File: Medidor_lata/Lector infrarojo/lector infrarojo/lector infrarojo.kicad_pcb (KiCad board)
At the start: 2 copper layers, 70 x 23 mm, 22 parts, among them J1 Conn_01x02_Female, J2 Conn_01x02_Female

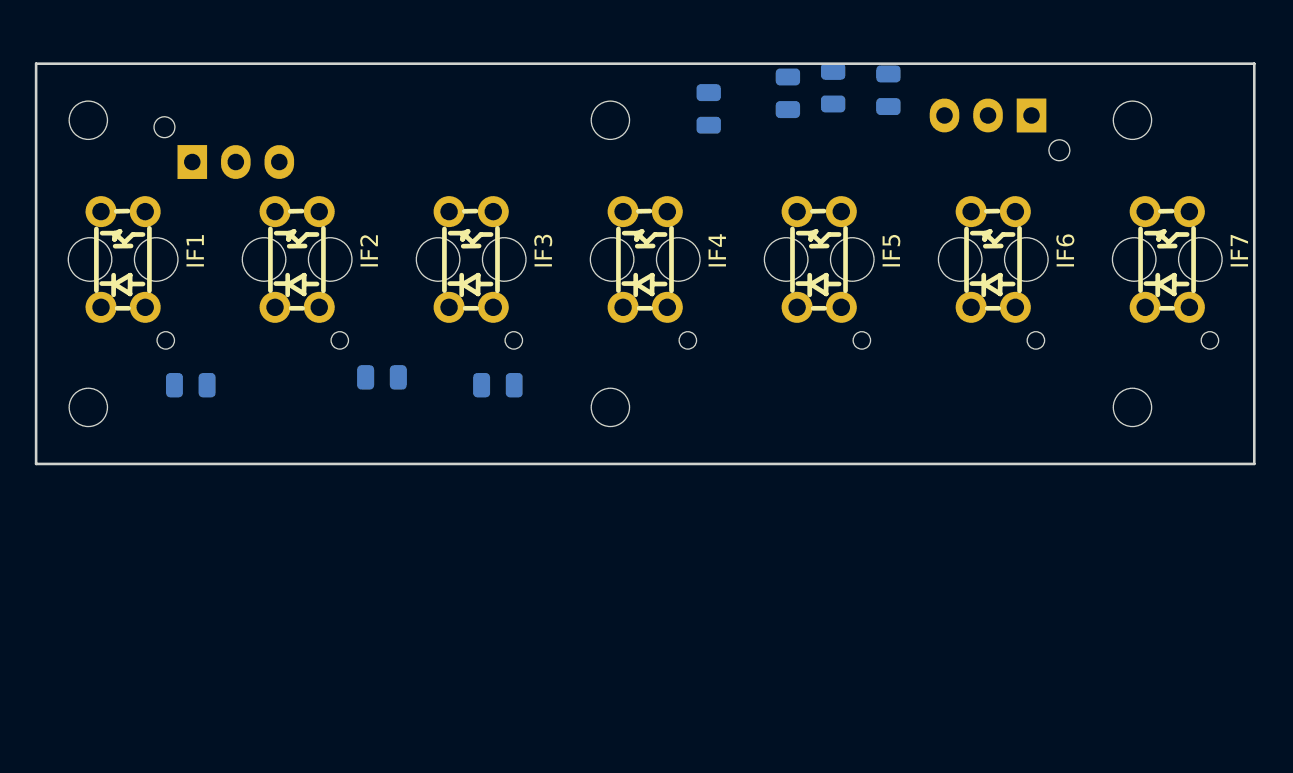
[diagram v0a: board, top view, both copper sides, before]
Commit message: Cambios de medidor
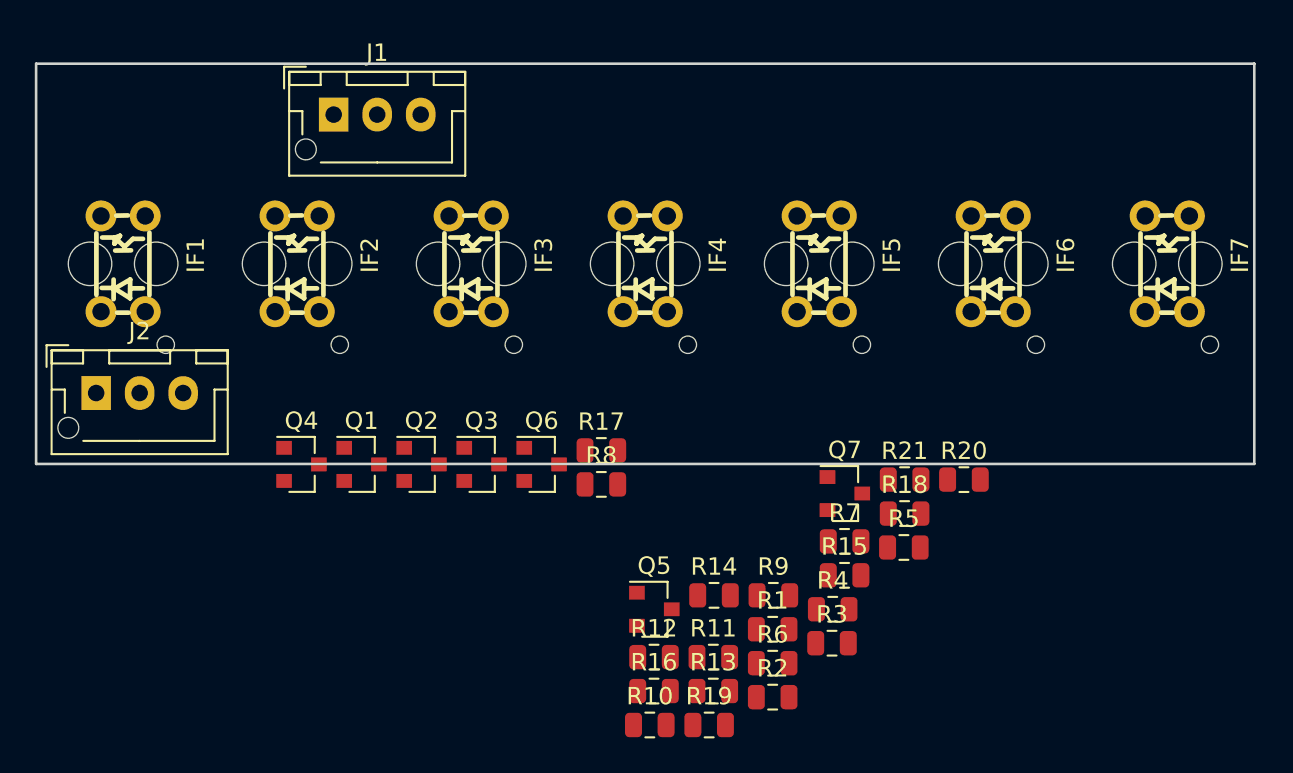
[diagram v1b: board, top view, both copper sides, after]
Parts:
- removed REF** (x6): MountingHole_2.2mm_M2, MountingHole:MountingHole_2.2mm_M2
- added Q1: BC857, Package_TO_SOT_SMD:SOT-23, F.Cu at (118.7, 101.8)
- added Q2: BC857, Package_TO_SOT_SMD:SOT-23, F.Cu at (122.2, 101.8)
- added Q3: BC857, Package_TO_SOT_SMD:SOT-23, F.Cu at (125.6, 101.8)
- added Q4: BC857, Package_TO_SOT_SMD:SOT-23, F.Cu at (115.3, 101.8)
- added Q5: BC857, Package_TO_SOT_SMD:SOT-23, F.Cu at (135.5, 110.1)
- added Q6: BC857, Package_TO_SOT_SMD:SOT-23, F.Cu at (129.1, 101.8)
- added Q7: BC857, Package_TO_SOT_SMD:SOT-23, F.Cu at (146.5, 103.5)
- added R10: R, Resistor_SMD:R_0805_2012Metric, F.Cu at (135.3, 116.8)
- added R11: R, Resistor_SMD:R_0805_2012Metric, F.Cu at (138.9, 112.9)
- added R12: R, Resistor_SMD:R_0805_2012Metric, F.Cu at (135.5, 112.9)
- added R13: R, Resistor_SMD:R_0805_2012Metric, F.Cu at (138.9, 114.8)
- added R14: R, Resistor_SMD:R_0805_2012Metric, F.Cu at (139.0, 109.3)
- added R15: R, Resistor_SMD:R_0805_2012Metric, F.Cu at (146.5, 108.2)
- added R16: R, Resistor_SMD:R_0805_2012Metric, F.Cu at (135.5, 114.8)
- added R17: R, Resistor_SMD:R_0805_2012Metric, F.Cu at (132.5, 101.0)
- added R18: R, Resistor_SMD:R_0805_2012Metric, F.Cu at (149.9, 104.6)
- added R19: R, Resistor_SMD:R_0805_2012Metric, F.Cu at (138.7, 116.8)
- added R20: R, Resistor_SMD:R_0805_2012Metric, F.Cu at (153.3, 102.7)
- added R21: R, Resistor_SMD:R_0805_2012Metric, F.Cu at (149.9, 102.7)
- added R8: R, Resistor_SMD:R_0805_2012Metric, F.Cu at (132.5, 102.9)
- added R9: R, Resistor_SMD:R_0805_2012Metric, F.Cu at (142.4, 109.3)
- J1, J2, R1, R2, R3, R4, R5, R6, R7: moved to F.Cu
- moved J2 56.1 mm to (103.5, 97.7), turned to 0 degrees
- moved R1 36.3 mm to (142.3, 111.3)
- moved R6 33.3 mm to (142.3, 113.2), turned to 0 degrees
- moved R4 29.6 mm to (145.8, 110.1), turned to 0 degrees
- moved R2 29.0 mm to (142.3, 115.2)
- moved R5 26.9 mm to (149.9, 106.6), turned to 0 degrees
- moved R7 26.0 mm to (146.5, 106.2), turned to 0 degrees
- moved R3 24.3 mm to (145.7, 112.1)
- moved J1 8.57 mm to (117.1, 81.7)
- moved IF1 0.25 mm to (105.0, 90.2)
- moved IF2 0.25 mm to (115.0, 90.2)
- moved IF3 0.25 mm to (125.0, 90.2)
- moved IF4 0.25 mm to (135.0, 90.2)
- moved IF5 0.25 mm to (145.0, 90.2)
- moved IF6 0.25 mm to (155.0, 90.2)
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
